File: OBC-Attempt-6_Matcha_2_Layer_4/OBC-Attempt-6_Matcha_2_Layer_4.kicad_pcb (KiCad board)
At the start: 2 copper layers, 57.1 x 57.1 mm, 59 parts, among them J2 Screw_Terminal_01x08, J3 Screw_Terminal_01x08, J5 Conn_01x04, J6 Micro_SD_Card, J7 Screw_Terminal_01x02, J8 Screw_Terminal_01x02, SW1 PCM12SMTR, U1 BMI088, U10 CPC1020NTR, U11 CPC1020NTR, U12 NCP1117-3.3_SOT223, U2 CPC1020NTR, U3 CPC1020NTR, U4 CPC1020NTR, U5 CPC1020NTR, U7 CPC1020NTR, U8 CPC1020NTR, U9 STM32F401RDTx, Y1 ABMM2-25MHZ-D1-T

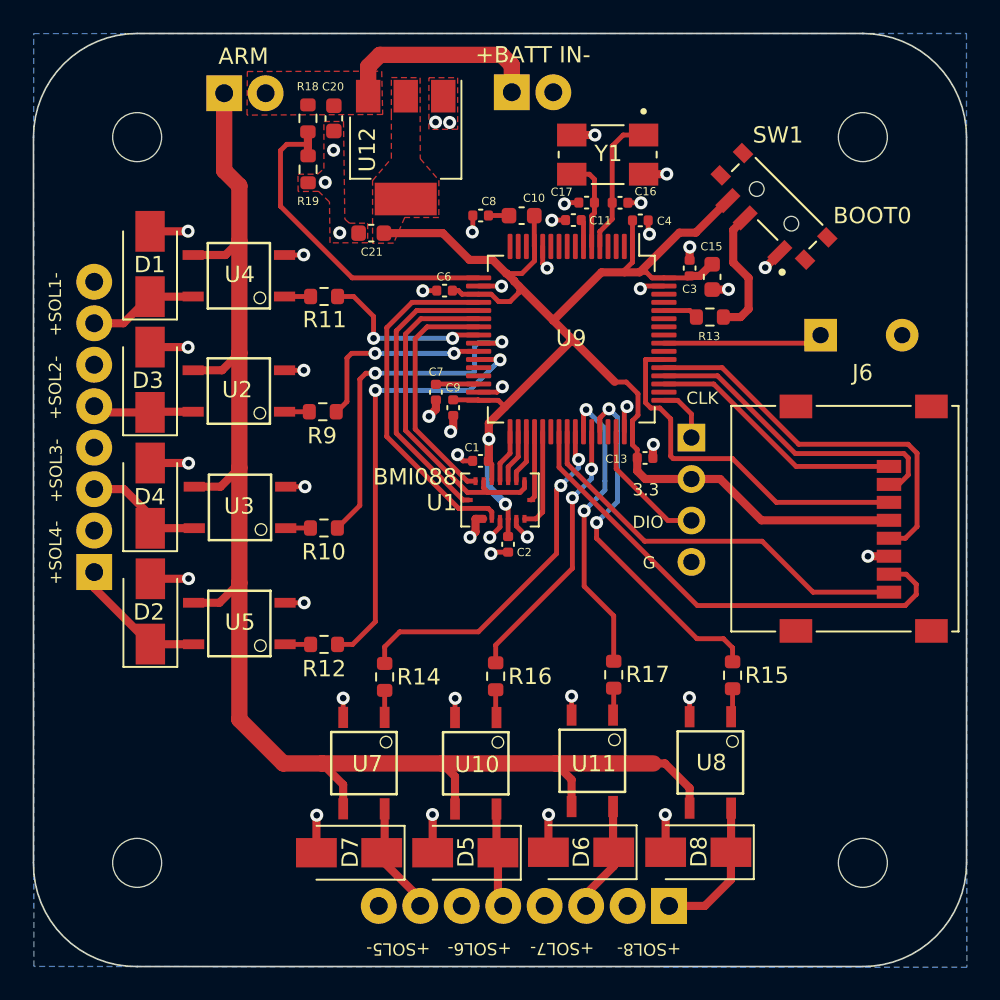
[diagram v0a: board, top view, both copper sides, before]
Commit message: Some Changes
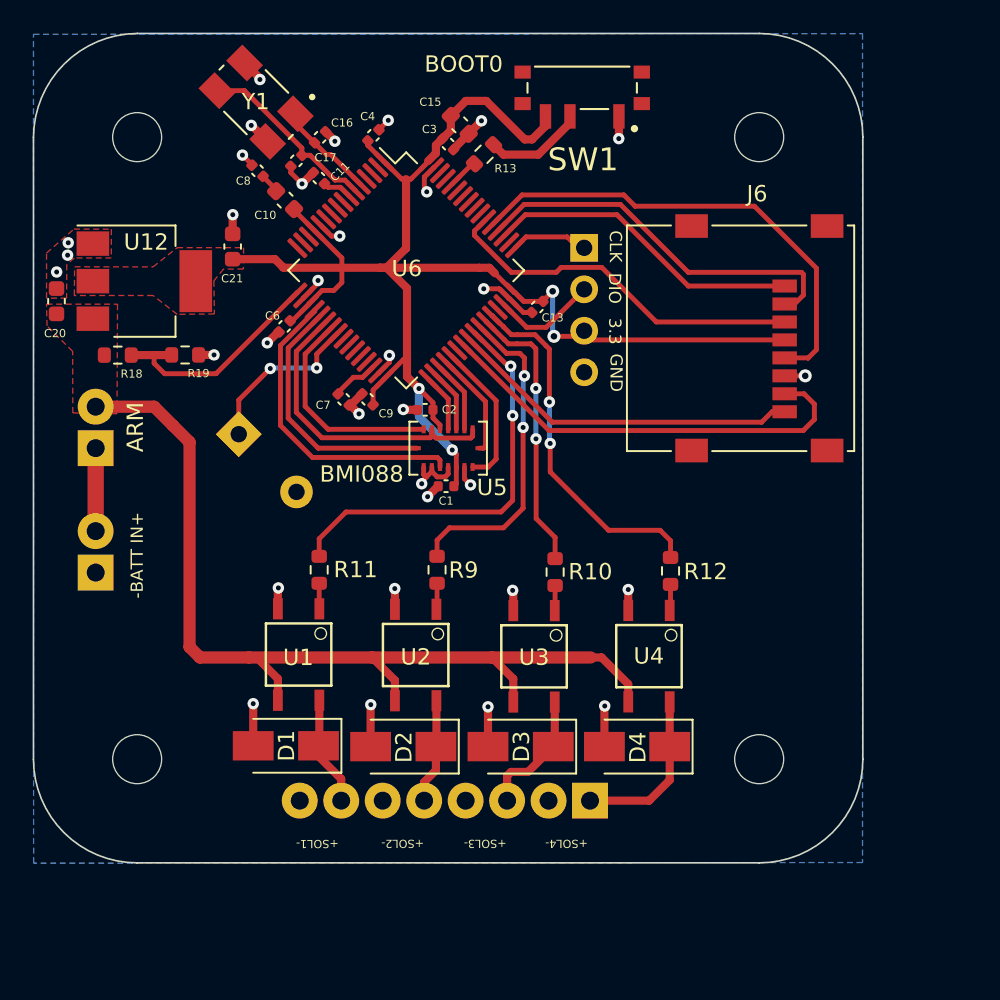
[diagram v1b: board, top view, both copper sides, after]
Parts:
- removed D5, D6, D7, D8: B330, Diode_SMD:D_SMA
- removed J3: Screw_Terminal_01x08, TerminalBlock_Phoenix:TerminalBlock_Phoenix_MPT-0,5-8-2.54_1x08_P2.54mm_Horizontal
- removed R14, R15, R16, R17: 270, Resistor_SMD:R_0603_1608Metric
- removed U10, U11, U7, U8: CPC1020NTR, CPC1020NTR:4-SOP
- moved J7 38.9 mm to (29.2, 58.4), turned to 90 degrees
- moved BZ1 36.1 mm to (38.0, 49.9), turned to -45 degrees
- moved J2 33.4 mm to (59.5, 72.4), turned to 180 degrees
- moved D4 30.9 mm to (62.4, 69.1), turned to 180 degrees
- moved D1 30.7 mm to (40.9, 69.0), turned to 180 degrees
- moved D3 27.4 mm to (55.2, 69.1), turned to 180 degrees
- moved D2 27.3 mm to (48.0, 69.1), turned to 180 degrees
- moved U4 25.2 mm to (63.1, 63.5), turned to 180 degrees
- moved U1 23.5 mm to (41.6, 63.4), turned to 180 degrees
- moved J8 23.1 mm to (29.2, 50.8), turned to 90 degrees
- moved Y1 21.8 mm to (39.0, 29.6), turned to -135 degrees
- moved R12 21.7 mm to (64.4, 58.3), turned to 90 degrees
- moved C20 20.3 mm to (26.8, 41.8), turned to 90 degrees
- moved U3 20.2 mm to (56.1, 63.5), turned to 180 degrees
- moved U2 19.5 mm to (48.8, 63.5), turned to 180 degrees
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- renumbered D3 to D2, D4 to D3, D2 to D4, U4 to U1, U5 to U4, U1 to U5, U9 to U6
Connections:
- C20 pad 1: BATT+ -> PWR
- J5 pad 2: 3.3V -> SYS_JTMS-SWDIO
- J5 pad 3: SYS_JTMS-SWDIO -> 3.3V
- J7 pad 1: BATT+ -> GND
- J7 pad 2: GND -> BATT+
- J8 pad 1: PWR -> BATT+
- J8 pad 2: BATT+ -> PWR
- R18 pad 1: BATT+ -> PWR
- U12 pad 3: BATT+ -> PWR
- U6 pad 24: SOL1 -> BUZZER
- U6 pad 25: SOL3 -> unconnected-(U6-Pad25)
- U6 pad 26: SOL2 -> unconnected-(U6-Pad26)
- U6 pad 27: SOL4 -> unconnected-(U6-Pad27)
- U6 pad 41: SOL5 -> SOL1
- U6 pad 42: SOL7 -> SOL2
- U6 pad 43: SOL6 -> SOL3
- U6 pad 44: SOL8 -> SOL4
- U6 pad 56: BUZZER -> unconnected-(U6-Pad56)
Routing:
- net PWR: track 91.8 -> 58.2 mm
- net SOL8: track 22.3 -> 0.00 mm, vias 2 -> 0
- net SOL5: track 22.0 -> 0.00 mm, vias 2 -> 0
- net SOL7: track 18.6 -> 0.00 mm, vias 2 -> 0
- net SOL6: track 16.6 -> 0.00 mm, vias 2 -> 0
- net SOL1: track 10.6 -> 25.2 mm
- net Net-(D8-Pad1): track 8.85 -> 0.00 mm
- net GND: track 57.9 -> 49.3 mm, vias 46 -> 33
- net SOL2: track 11.8 -> 19.8 mm
- net BATT+: track 12.8 -> 5.08 mm
- net Net-(D7-Pad1): track 7.00 -> 0.00 mm
- net Net-(D6-Pad1): track 6.80 -> 0.00 mm
- net VMON: track 20.7 -> 14.1 mm
- net Net-(D5-Pad1): track 6.11 -> 0.00 mm
- net RCC_OSC_OUT: track 5.70 -> 11.3 mm
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- added copper zone on F.Cu, net PWR
- removed copper zone on F.Cu, net BATT+
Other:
- board size 57.1 x 57.1 mm -> 50.8 x 50.8 mm
- board text added: "-BATT IN+"
- board text added: "GND"
- board text added: "MATCHA V2.0"
- board text removed: "+BATT IN-"
- board text removed: "+SOL5-"
- board text removed: "+SOL6-"
- board text removed: "+SOL7-"
- board text removed: "+SOL8-"
- board text removed: "G"
- board text removed: "MATCHA V3.0"
